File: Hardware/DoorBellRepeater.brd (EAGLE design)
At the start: 65.7 x 36.8 mm, 25 parts, among them IC1 LM1117

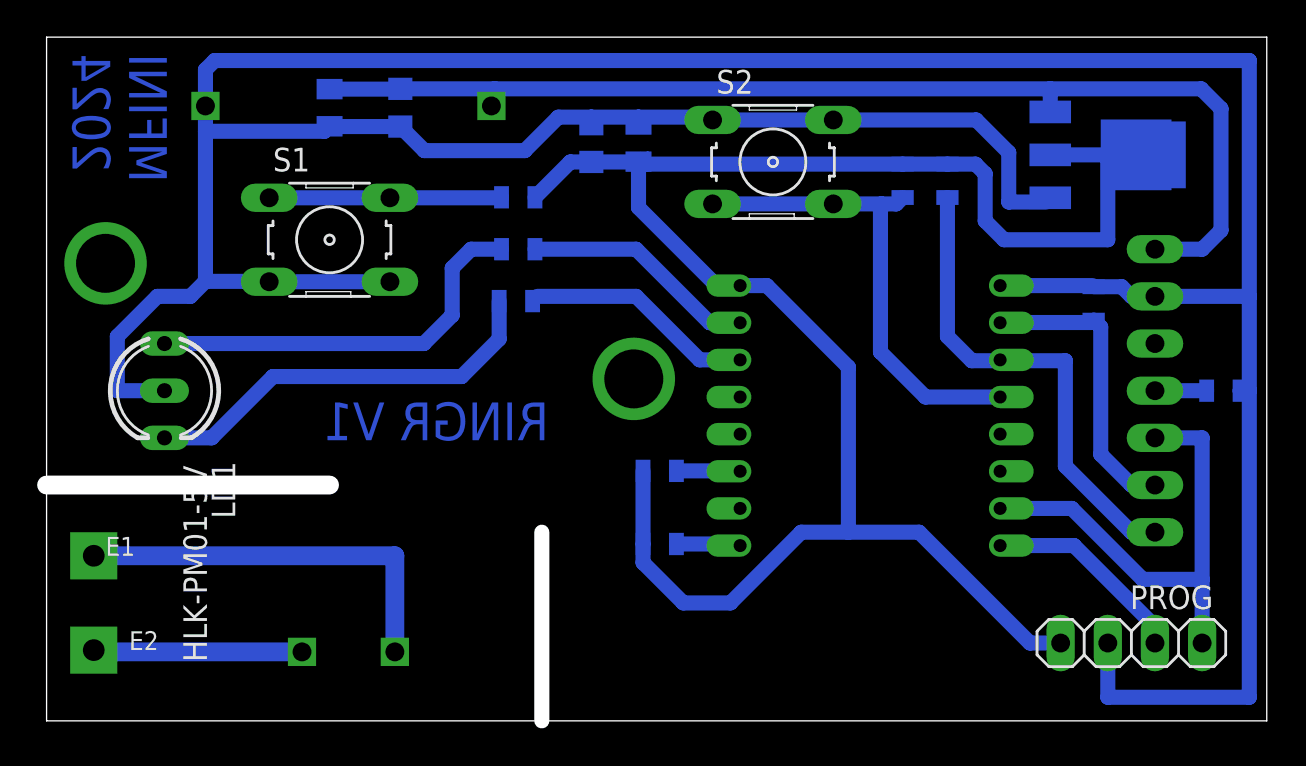
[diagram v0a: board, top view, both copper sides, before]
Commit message: Add files via upload
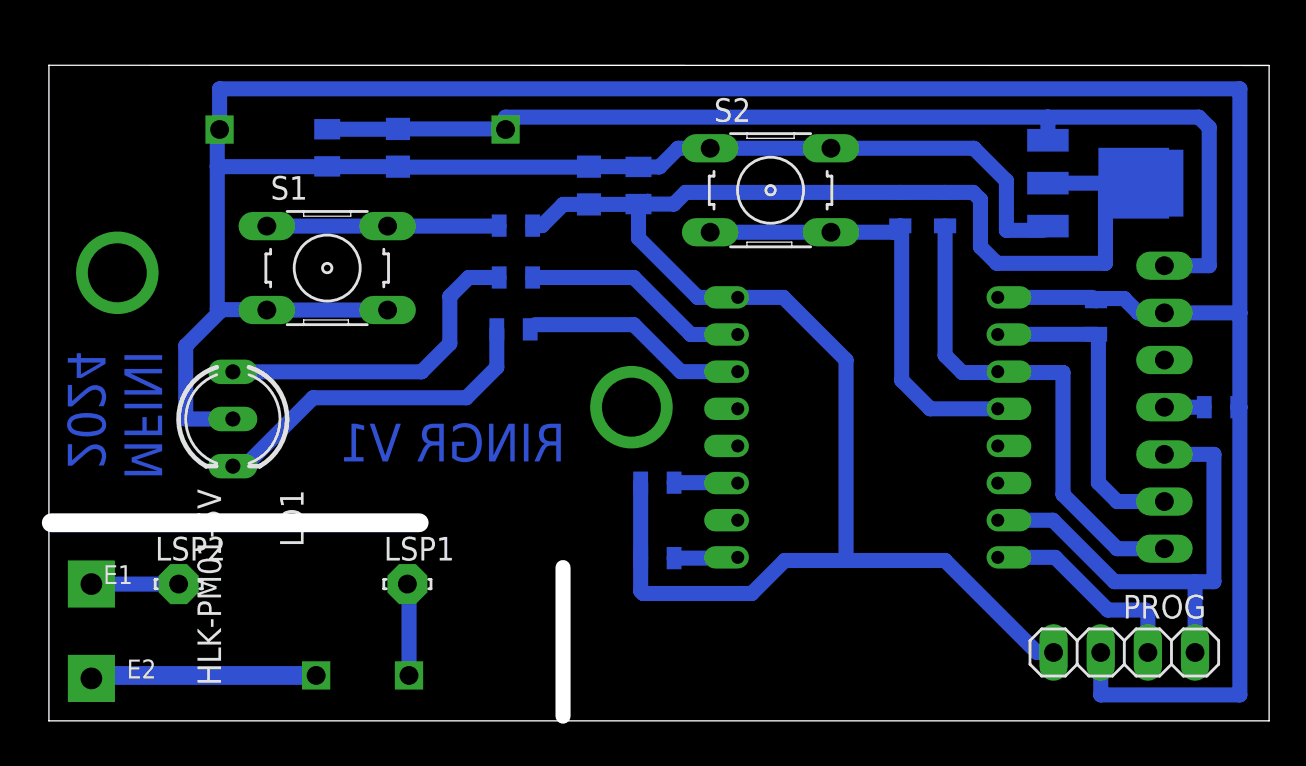
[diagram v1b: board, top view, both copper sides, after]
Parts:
- added LSP1, LSP2: LSP10, solpad:LSP10
- moved LD1 3.99 mm to (10.0, 16.3)
- moved C2 2.29 mm to (29.2, 28.8)
- moved C23 2.29 mm to (31.9, 28.8)
- moved C1 2.16 mm to (18.9, 30.9)
- moved C3 2.16 mm to (15.1, 30.9)
- moved MGT2 1.53 mm to (31.5, 16.9)
- moved S2 1.53 mm to (39.0, 28.6)
- moved E1 1.53 mm to (2.41, 7.37)
- moved IC1 1.53 mm to (57.0, 29.0)
- moved R8 1.53 mm to (25.1, 21.1)
- moved S1 1.53 mm to (15.1, 24.4)
- moved E2 1.53 mm to (2.41, 2.29)
- moved R5 1.53 mm to (46.0, 27.6)
- moved R6 1.53 mm to (48.4, 27.6)
- moved R2 1.53 mm to (25.3, 26.7)
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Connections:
- new net N$2: HLK-PM01-5V.P$2, LSP1.MP
- net N$6: now also LSP2.MP; no longer HLK-PM01-5V.P$2
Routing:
- net N$6: track 21.4 -> 4.70 mm
- net GND: track 199.4 -> 190.2 mm
- net N$2: track 0.00 -> 4.96 mm
- net N$4: track 22.3 -> 18.5 mm
- net N$5: track 21.7 -> 17.9 mm
- net 5V: track 61.3 -> 59.6 mm
- net 3V3: track 102.2 -> 100.5 mm
- net LRC: track 26.4 -> 28.0 mm
- net GPIO0: track 26.0 -> 24.7 mm
- net BCLK: track 16.1 -> 17.3 mm
- net N$1: track 11.3 -> 12.2 mm
- net GAIN: track 2.78 -> 2.15 mm
- net TX: track 11.4 -> 12.0 mm
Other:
- board size 65.7 x 36.8 mm -> 65.7 x 35.3 mm
